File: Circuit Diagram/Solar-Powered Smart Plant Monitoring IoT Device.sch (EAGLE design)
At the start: 89 parts, among them J1 4-1437652-0, J10 FLASHER, J2 Nutrition Sensor, Q10 MMBT3904, Q13 AO3401, Q4 FS8205, Q5 AO3400-5.8A, Q9 MMBT3904, U1 CH340K, U2 LT3652HVEMSE#TRPBF, U4 DW01A, U5 CH340K

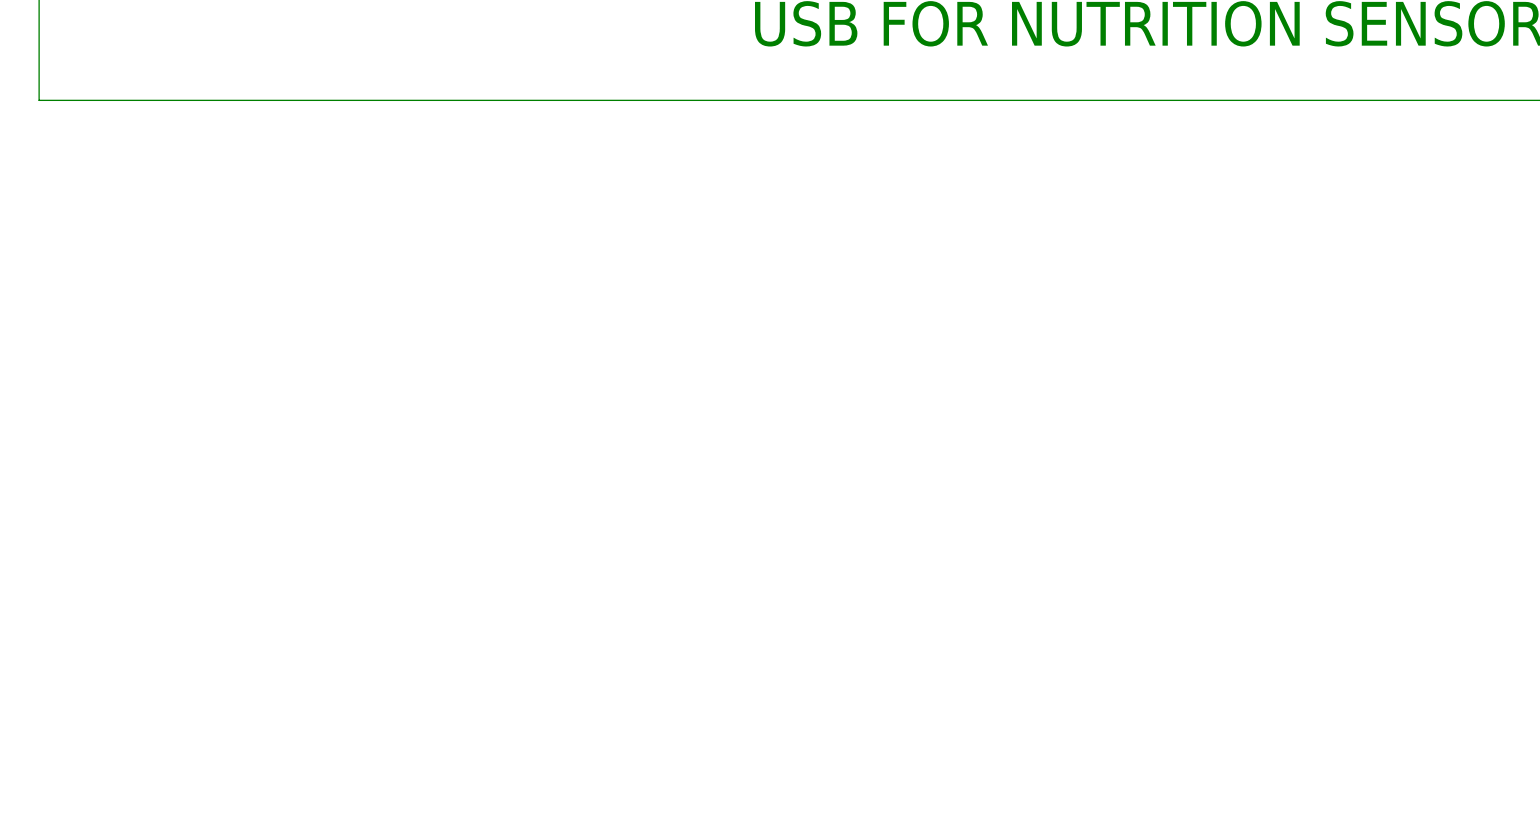
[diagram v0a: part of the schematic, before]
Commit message: Change readme.md and edit sch
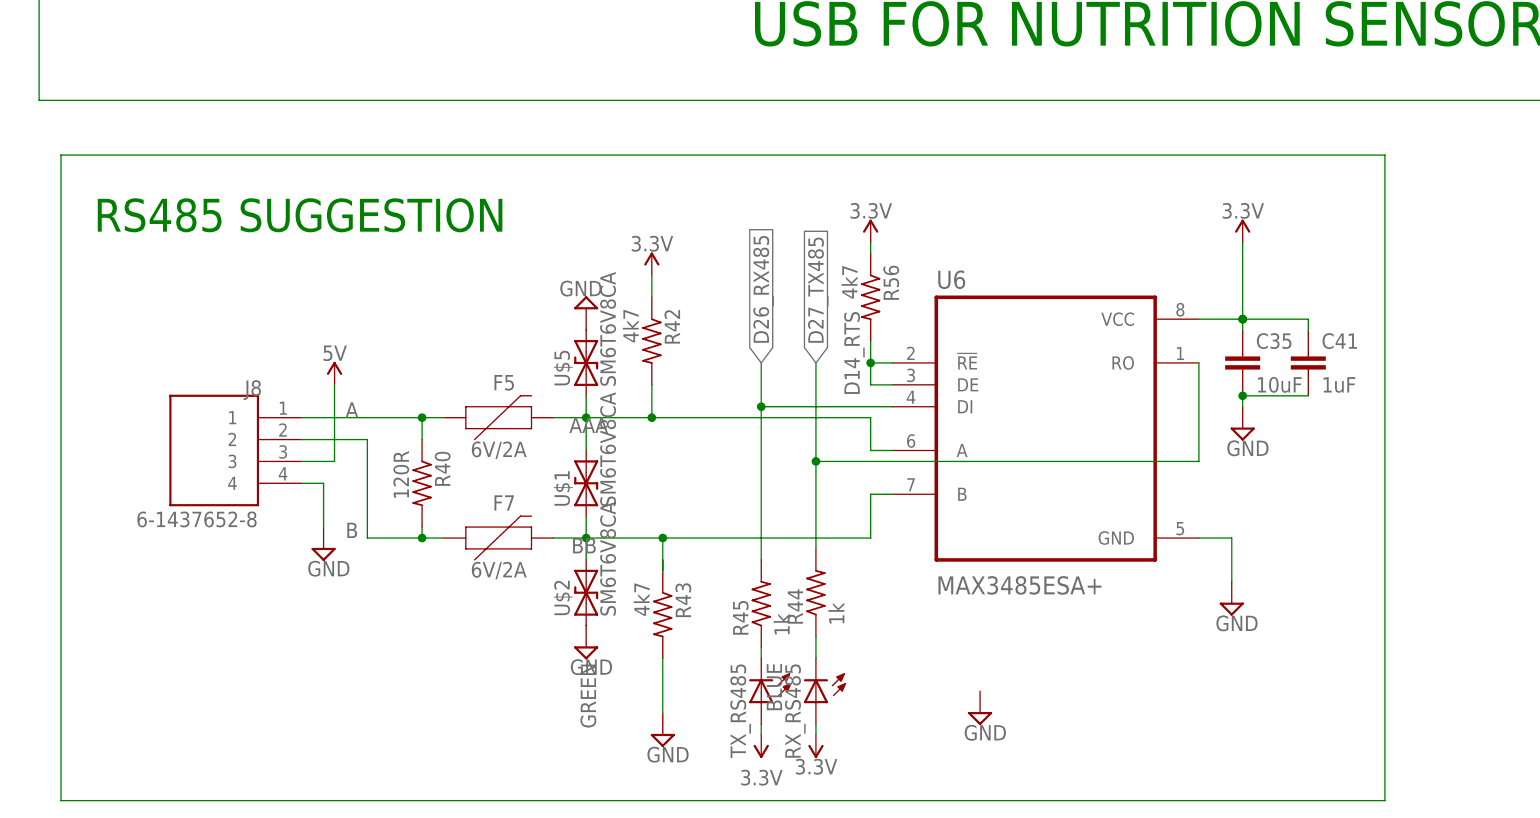
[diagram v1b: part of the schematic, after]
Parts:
- added C35: 10uF, rcl:C-EUC0603
- added C41: 1uF, rcl:C-EUC0603
- added F5, F7: 6V/2A, SparkFun-Fuses:PPTC_6V2A
- added J8: 6-1437652-8, 6-1437652-8:6-1437652-8
- added R40: 120R, adafruit:R-US_R0603
- added R42, R43, R56: 4k7, adafruit:R-US_R0603
- added R44, R45: 1k, adafruit:R-US_R0603
- added RX_RS485: BLUE, adafruit:LEDCHIP-LED0603
- added TX_RS485: GREEN, adafruit:LEDCHIP-LED0603
- added U$1, U$2, U$5: SM6T6V8CA, SM6T6V8CA:SM6T6V8CA
- added U6: MAX3485ESA+, MAX3485ESA_:MAX3485ESA+
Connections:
- new net A: F5.1, J8.1, R40.1
- new net AAA: F5.2, R42.2, U$1.2, U$5.1, U6.A
- new net B: F7.1, J8.2, R40.2
- new net BB: F7.2, R43.1, U$1.1, U$2.2, U6.B
- new net N$46: R44.1, RX_RS485.C
- new net N$47: R45.1, TX_RS485.C
- net 3.3V: now also C35.1, C41.1, R42.1, R56.1, RX_RS485.A, TX_RS485.A, U6.VCC
- net 5V: now also J8.3
- net D14_RTS: now also R56.2, U6.!RE, U6.DE
- net D26_RX485: now also R45.2, U6.DI
- net D27_TX485: now also R44.2, U6.RO
- net GND: now also C35.2, C41.2, J8.4, R43.2, U$2.1, U$5.2, U6.GND
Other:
- note added: "RS485 SUGGESTION"
